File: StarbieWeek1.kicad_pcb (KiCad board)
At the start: 2 copper layers, 133 x 111 mm, 7 parts, among them J1 Conn_01x04_Pin, J2 Conn_01x08_Pin, SW1 SW_Push, SW2 SW_Push, U1 XIAO-ESP32-C3-SMD, U2 DHT11

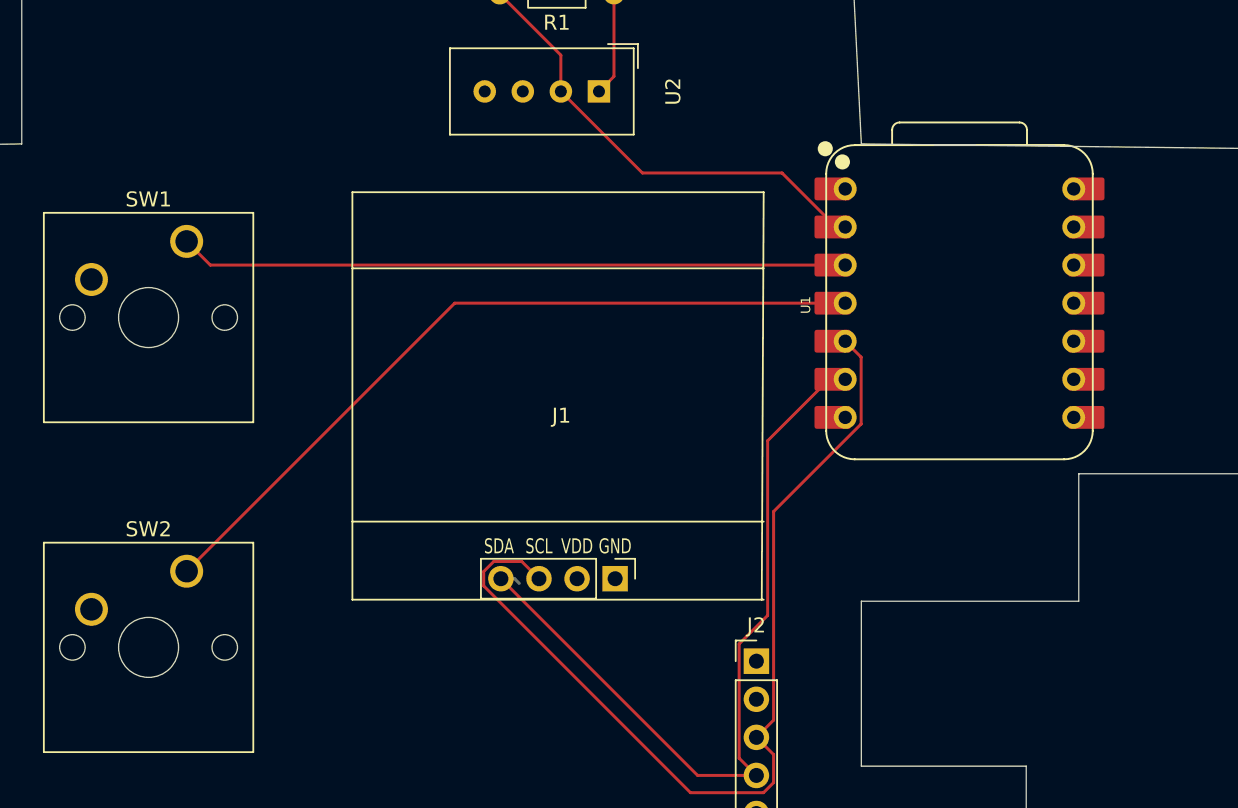
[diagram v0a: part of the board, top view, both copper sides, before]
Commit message: Update StarbieWeek1.kicad_pcb
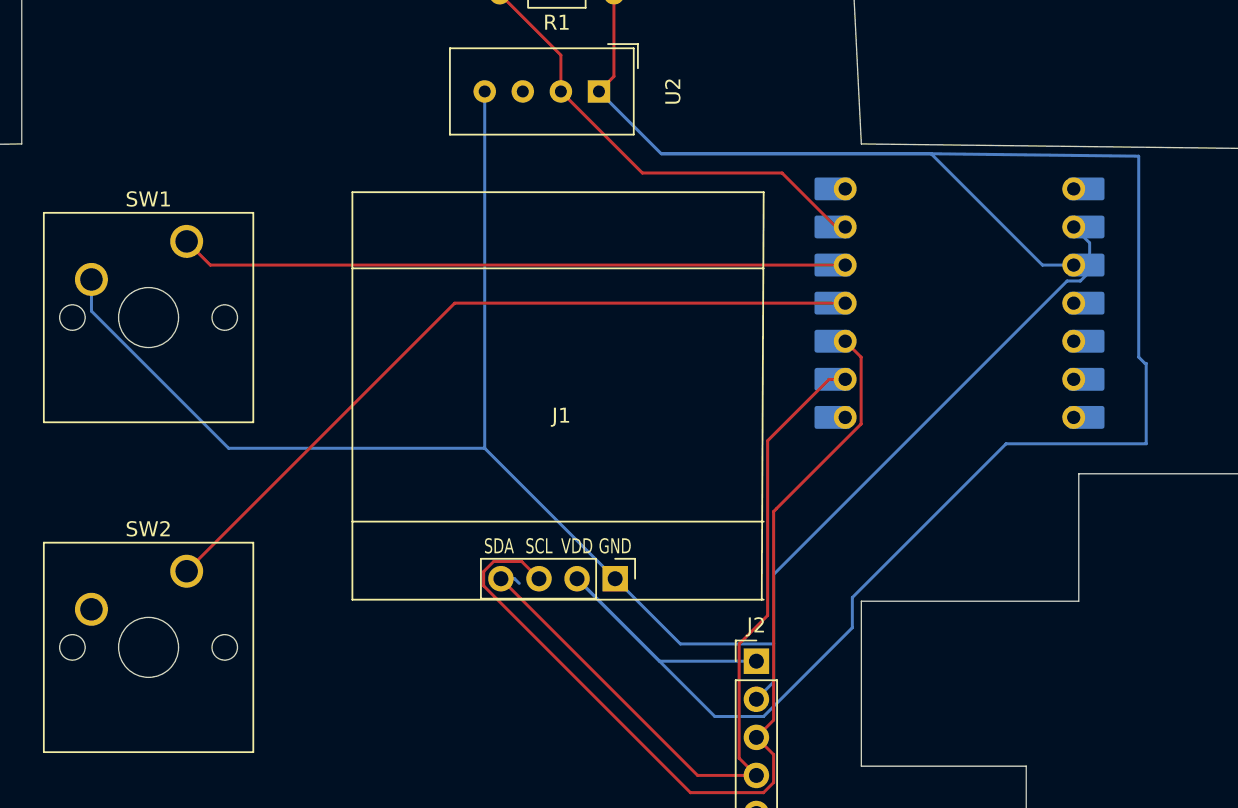
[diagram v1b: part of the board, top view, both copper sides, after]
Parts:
- U1: moved to B.Cu
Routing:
- net +3.3V: track 6.91 -> 159.4 mm
- net GND: track 0.00 -> 122.3 mm
